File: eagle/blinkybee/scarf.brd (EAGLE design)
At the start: 40 x 74 mm, 17 parts, among them IC1 TLC272P, M1 ELECTRET_MICROPHON-WM.64PN

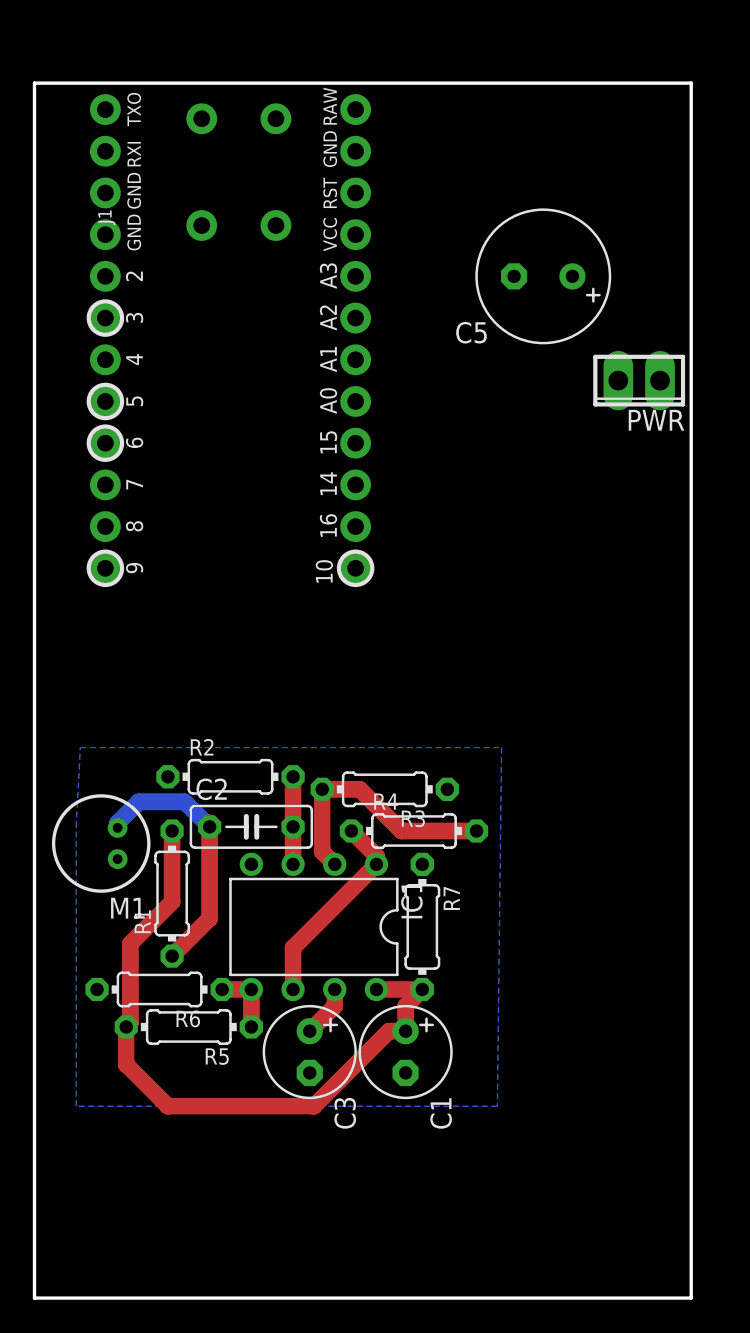
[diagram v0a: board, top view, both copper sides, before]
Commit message: scarf pcb
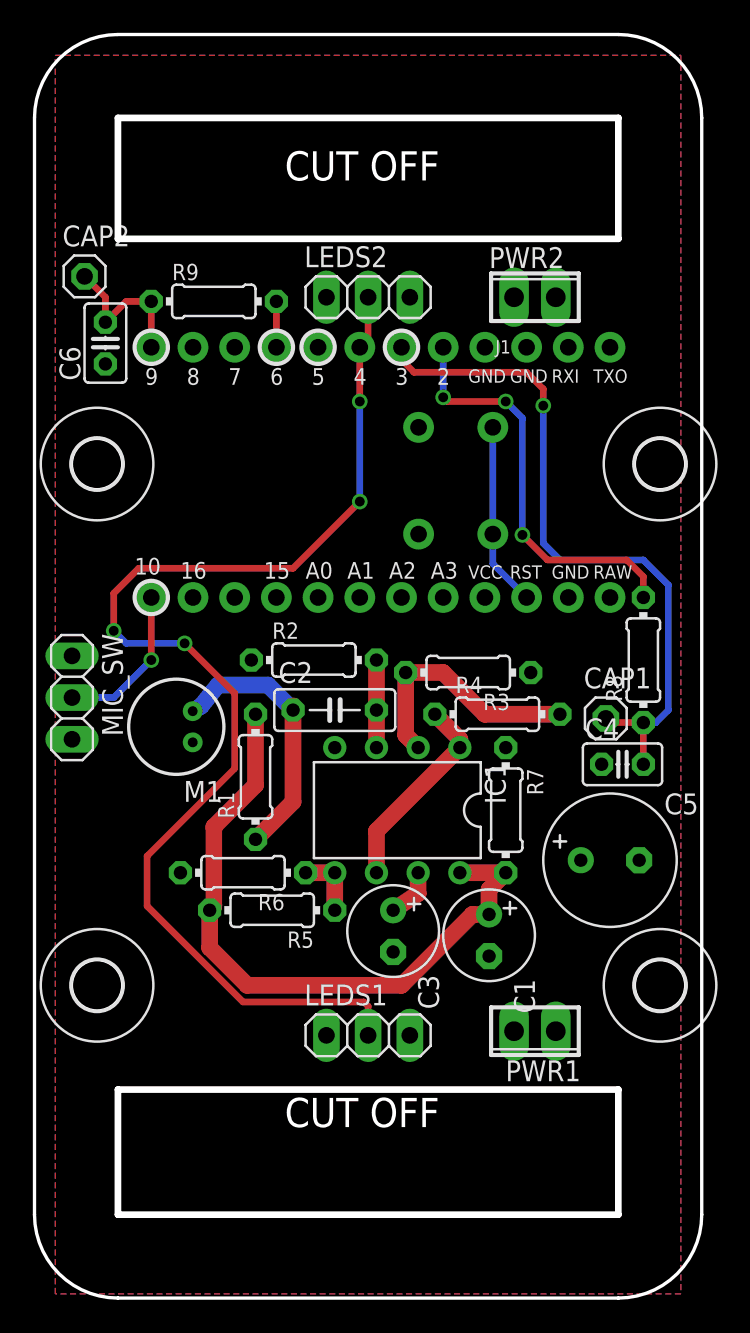
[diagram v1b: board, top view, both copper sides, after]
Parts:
- removed PWR: (no value), con-phoenix-254:2POL254
- added C4, C6: 0.1uF, rcl:C025-025X050
- added CAP1, CAP2: (no value), pinhead:1X01
- added H1, H2, H3, H4: MOUNT-HOLE3.0, holes:3,0
- added LEDS1, LEDS2, MIC_SW: (no value), pinhead:1X03
- added PWR1, PWR2: (no value), con-phoenix-254:2POL254
- added R8, R9: 5M, rcl:0204/7
- moved C5 35.8 mm to (35.1, 26.7), turned to 0 degrees
- moved JP6 33.5 mm to (35.1, 42.7), turned to 0 degrees
- moved S1 23.0 mm to (25.7, 49.8)
- moved JP7 13.7 mm to (7.11, 57.9), turned to 180 degrees
- moved C3 8.95 mm to (21.8, 22.4)
- moved R3 8.74 mm to (26.4, 38.1)
- moved R7 8.74 mm to (28.7, 29.7)
- moved C2 8.74 mm to (18.3, 35.8)
- moved R1 8.74 mm to (13.5, 31.8)
- moved R2 8.74 mm to (17.0, 38.9)
- moved R4 8.74 mm to (28.2, 35.6)
- moved R5 8.74 mm to (14.5, 23.6)
- moved R6 8.74 mm to (12.7, 25.9)
- moved C1 8.74 mm to (27.7, 22.1)
- moved IC1 8.74 mm to (22.1, 29.7)
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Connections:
- net MIC_OUT renamed MIC_OUT_D
- net N$4 renamed MIC_OUT_A
- net D10: now also MIC_SW.2
- net D2: now also R8.2
- net D3: now also C4.2, CAP1.1, R8.1
- net D4: now also LEDS1.2, LEDS2.2
- net D6: now also R9.2
- net D9: now also C6.2, CAP2.1, R9.1
- net GND: now also C4.1, C6.1, LEDS1.1, LEDS2.1, MIC_SW.1, PWR1.2, PWR2.2; no longer PWR.2
- net VCC: now also LEDS1.3, LEDS2.3, MIC_SW.3, PWR1.1, PWR2.1; no longer PWR.1
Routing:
- net D4: track 0.00 -> 74.1 mm, vias 0 -> 4
- net D3: track 0.00 -> 42.6 mm, vias 0 -> 1
- net D2: track 0.00 -> 25.2 mm, vias 0 -> 3
- net RESET: track 0.00 -> 11.2 mm
- net D10: track 0.00 -> 9.58 mm, vias 0 -> 1
- net D9: track 0.00 -> 9.43 mm
- net D6: track 0.00 -> 2.79 mm
- added copper zone on layer 1, net VCC
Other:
- board size 40 x 74 mm -> 40.6 x 77 mm
- board text added: "CUT OFF"
